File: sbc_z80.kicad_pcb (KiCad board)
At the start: 4 copper layers, 102.6 x 50.8 mm, 95 parts, among them J1 RC80 Bus, J2 CTC Header, J3 AVR-JTAG-10, J4 IDE, J5 PIO Header, J6 Port A, J7 Port B, J8 USB_B_Micro, Q1 IRLML6402, SW1 Reset, U1 DS1813R-5+T&R, U10 Z84C2010AEG, U11 74HCT273, U12 MAX40200AUK, U2 AP7381-33SA, U3 CPU -Z84C0020AEG, U4 CTC - Z84C3010AEG, U5 CPLD - EPM7032STC44, U6 SRAM - IS62C5128BL-45TLI, U7 74HCT2G04, U8 SST39SF040, U9 SIO/3 - Z84C4310AEG, X1 CTX-636 50mhz

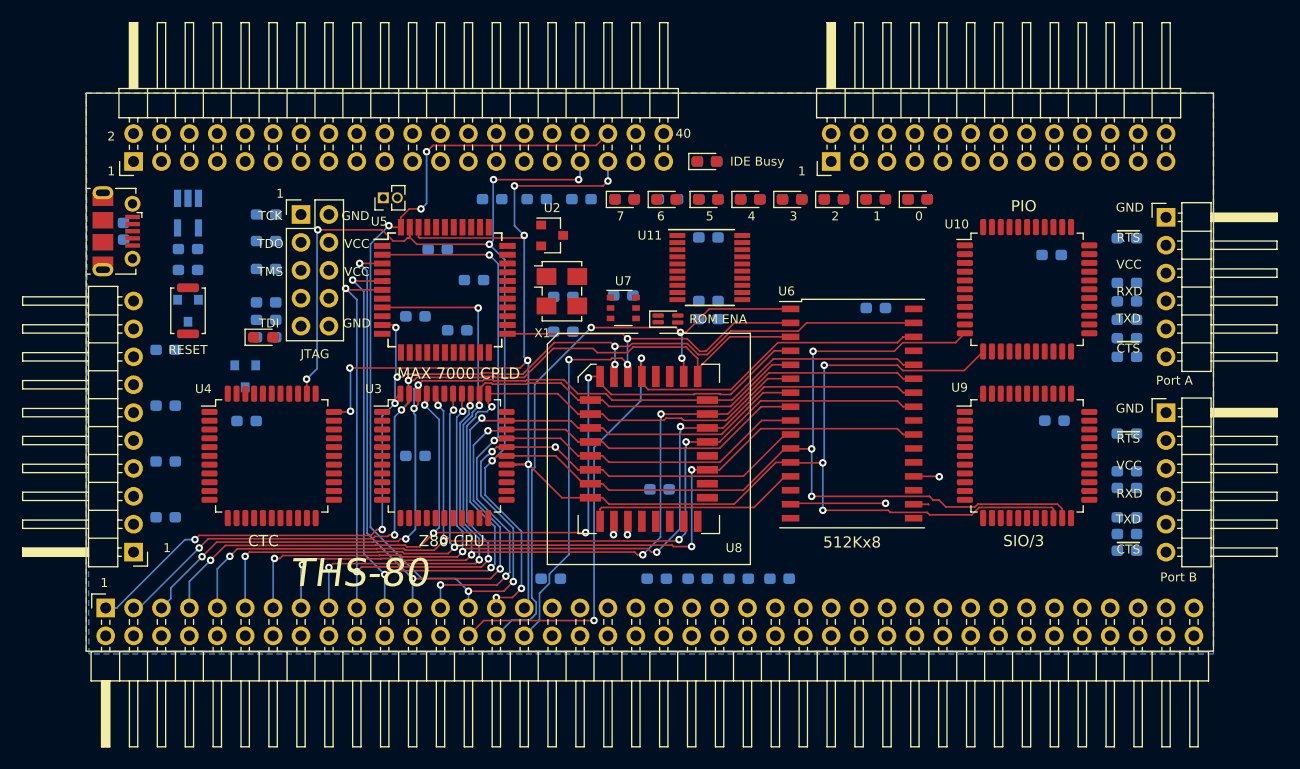
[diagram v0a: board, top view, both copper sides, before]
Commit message: more routing
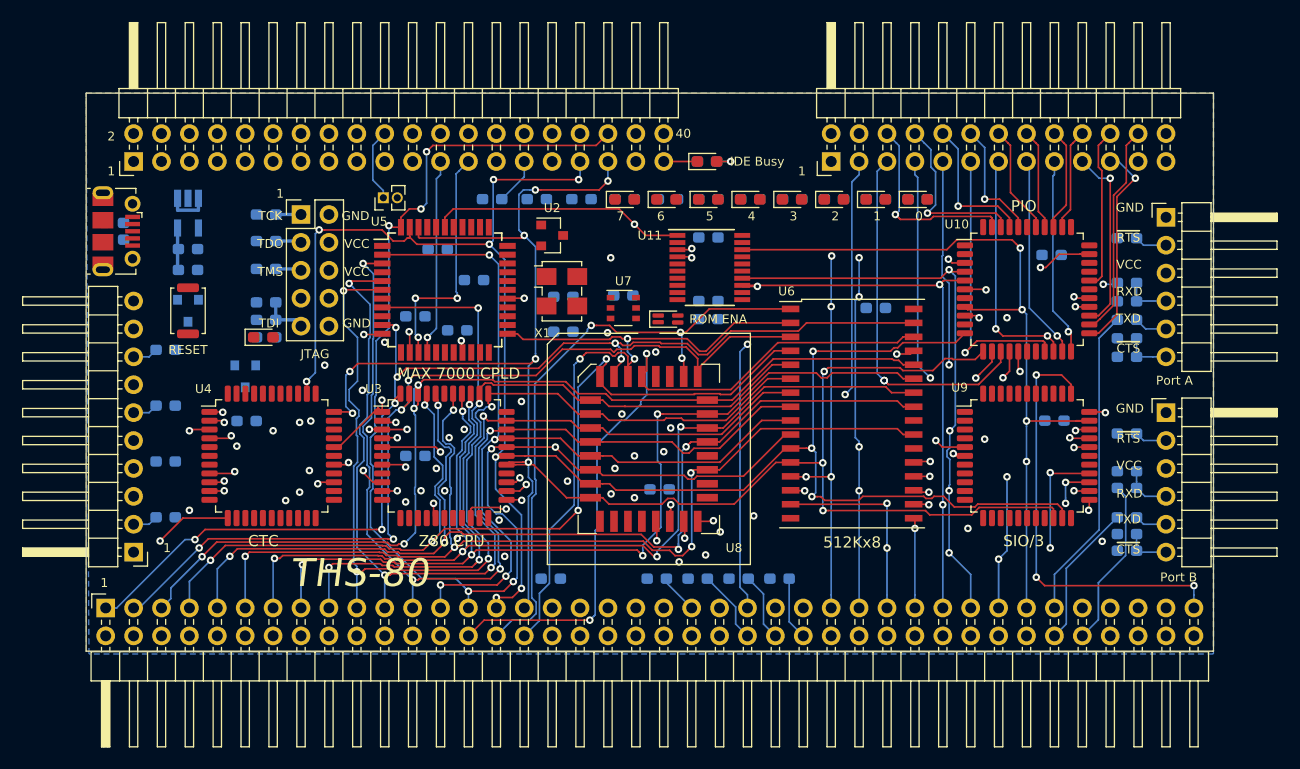
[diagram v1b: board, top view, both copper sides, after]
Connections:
- J1 pad 21: /CLK -> /CLK_CPU
- U3 pad 1: /CLK -> /CLK_CPU
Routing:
- net /D1: track 1.23 -> 186.7 mm, vias 1 -> 15
- net /D5: track 0.00 -> 179.5 mm, vias 0 -> 12
- net /D4: track 1.40 -> 170.8 mm, vias 0 -> 12
- net /D6: track 2.35 -> 168.4 mm, vias 1 -> 11
- net /IEI: track 0.00 -> 132.6 mm, vias 0 -> 6
- net /D7: track 0.00 -> 123.6 mm, vias 0 -> 6
- net /D3: track 0.00 -> 121.5 mm, vias 0 -> 12
- net /~M1: track 0.00 -> 114.5 mm, vias 0 -> 7
- net /D0: track 19.2 -> 121.3 mm, vias 0 -> 10
- net /~RESET: track 0.00 -> 101.2 mm, vias 0 -> 5
- net /D2: track 9.98 -> 110.8 mm, vias 2 -> 9
- net /CLK_CPU: track 0.00 -> 91.1 mm, vias 0 -> 6
- net /~IORQ: track 0.00 -> 75.4 mm, vias 0 -> 3
- net /~INT: track 0.00 -> 60.1 mm, vias 0 -> 3
- net /~WR: track 0.00 -> 58.1 mm, vias 0 -> 3
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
